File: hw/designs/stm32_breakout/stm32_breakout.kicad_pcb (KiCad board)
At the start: 2 copper layers, 15.2 x 33.8 mm, 16 parts, among them J1 USB_B_Micro, J2 Conn_01x10_Male, J3 Conn_01x10_Male, U1 AP7361C-33E, U2 STM32L031F6Px, U3 KC2016Z

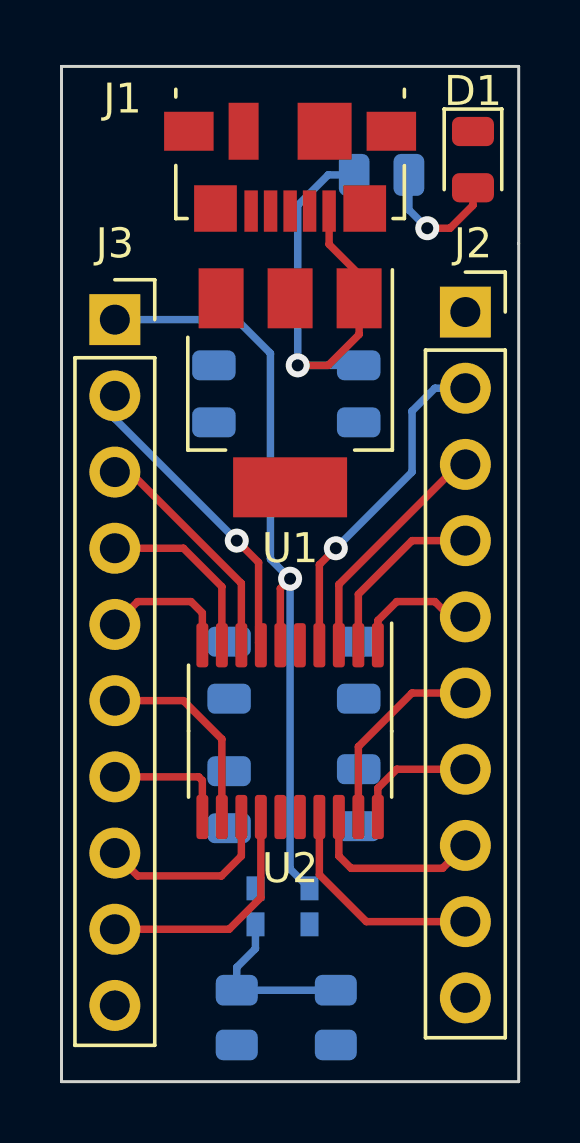
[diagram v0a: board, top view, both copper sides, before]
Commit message: Board is complete. Needs review
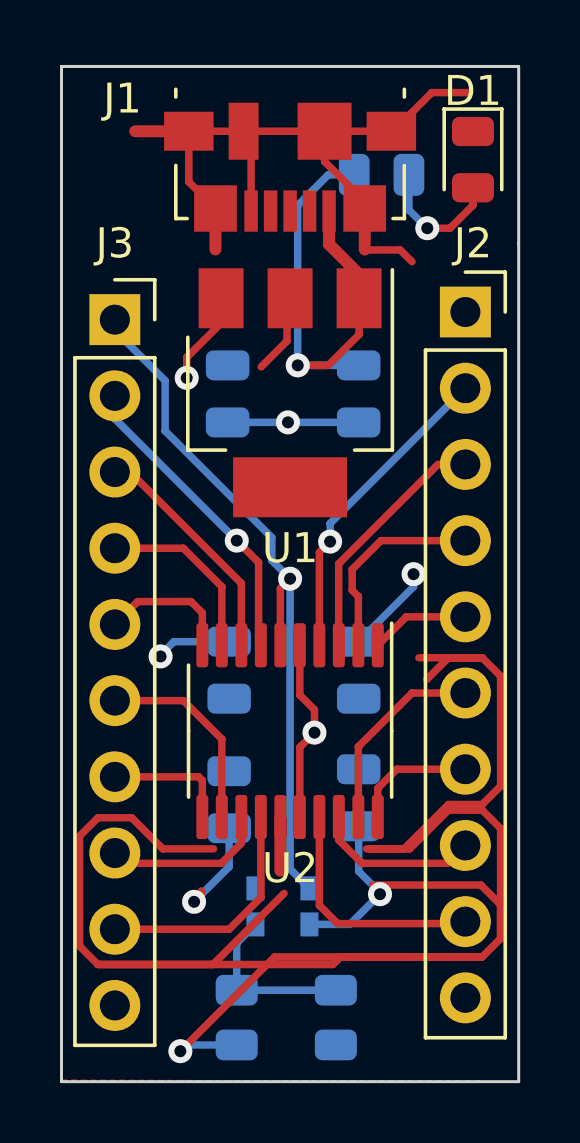
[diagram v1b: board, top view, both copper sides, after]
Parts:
- moved C2 0.46 mm to (130.0, 68.5)
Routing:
- net GND: track 0.00 -> 120.7 mm, vias 0 -> 6
- net +3V3: track 0.00 -> 9.26 mm, vias 0 -> 2
- net /PA0-CK_IN: track 26.4 -> 24.0 mm
- net /PB9-BOOT0: track 4.21 -> 3.31 mm
- net /PC14-OSC32IN: track 6.01 -> 6.78 mm
- net /PA9: track 7.44 -> 8.09 mm
- net /PA7: track 6.11 -> 5.51 mm
- net /NRST: track 11.2 -> 10.6 mm
- added copper zone on B.Cu, net +3V3
- added copper zone on F.Cu, net GND
